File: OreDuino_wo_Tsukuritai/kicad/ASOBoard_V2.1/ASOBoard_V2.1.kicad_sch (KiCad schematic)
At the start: 17 parts, among them SW1 SW_DIP_x01, U1 ATMega328P Arduino, U2 FT232RL, X1 Crystal 16MHz

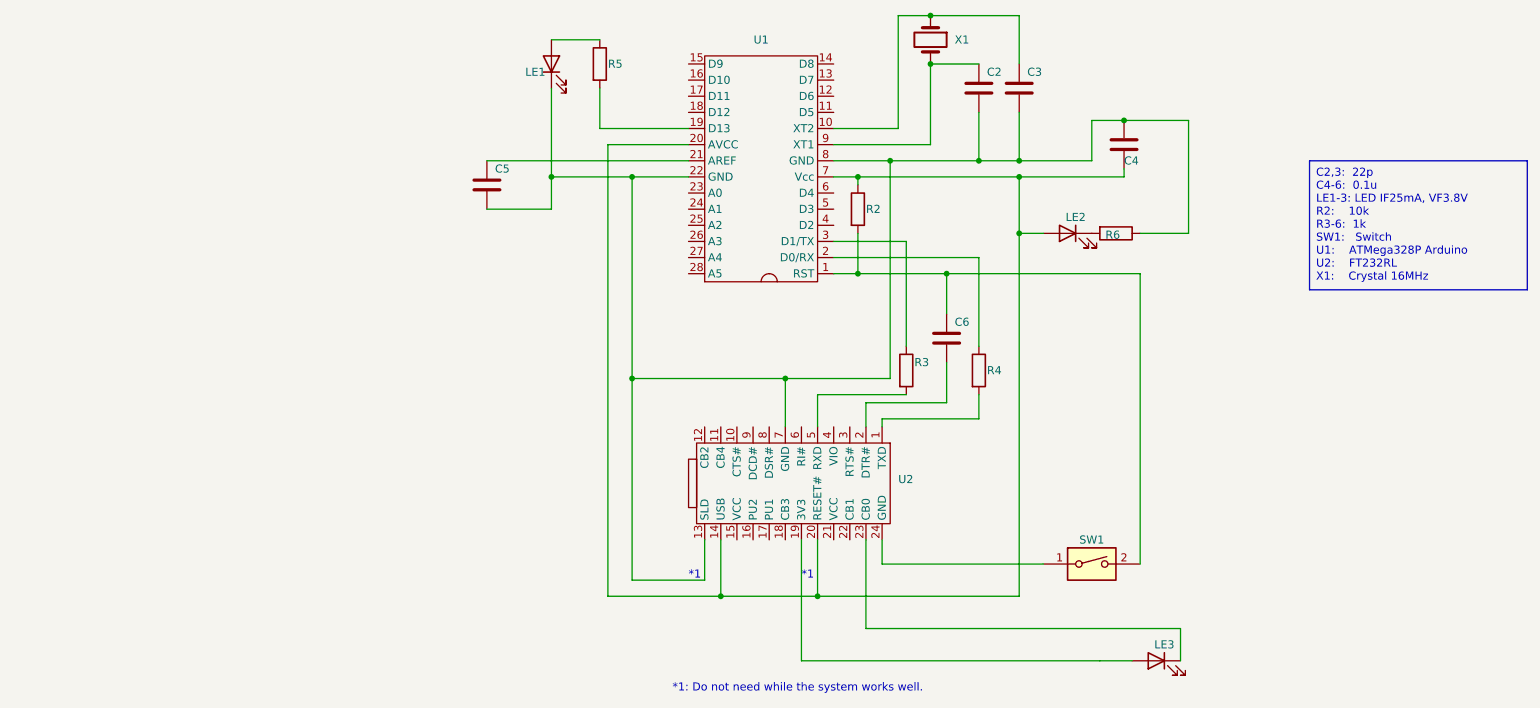
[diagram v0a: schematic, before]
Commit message: update
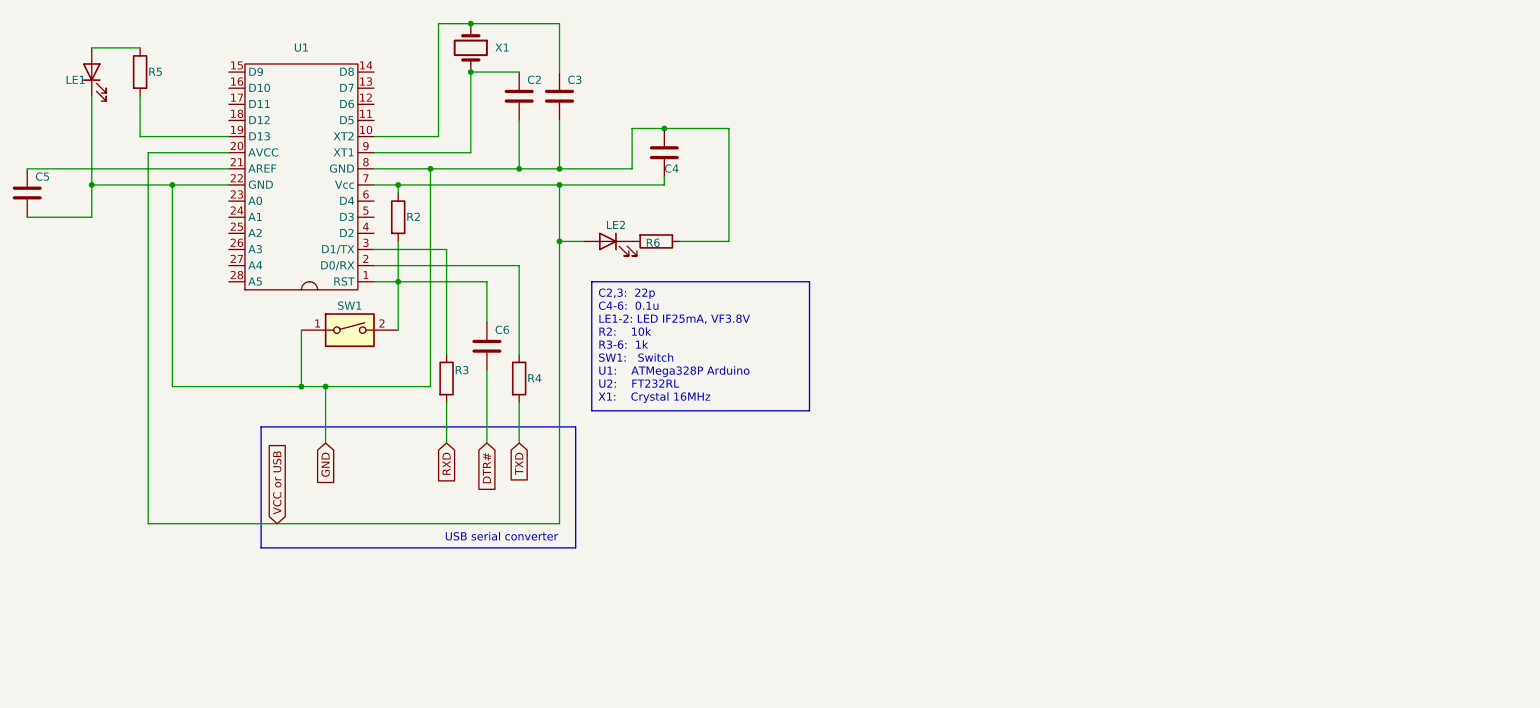
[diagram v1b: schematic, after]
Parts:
- removed LE3: LED IF25mA, VF3.8V, symbol Device:LED
- removed U2: FT232RL, symbol Ore:FT232RL_AKI
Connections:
- net GND: now reaches C2.2, C3.2, C4.1, C5.2, LE1.1 (K), R6.1, U1.22 (GND), U1.8 (GND)
- net GND: now also SW1.1
- net VCC or USB: now reaches C4.2, LE2.2 (A), R2.1, U1.20 (AVCC), U1.7 (Vcc)
- net TXD: now reaches R4.2
- net DTR#: now reaches C6.2
- net RXD: now reaches R3.2
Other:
- note added: "USB serial converter"
- note removed: "*1"
- note removed: "*1: Do not need while the system works well."
- moved on the sheet: C2, C3, C4, C5, C6, LE1, LE2, R2, R3, R4, R5, R6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
